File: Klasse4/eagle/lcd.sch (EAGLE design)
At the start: 3 parts

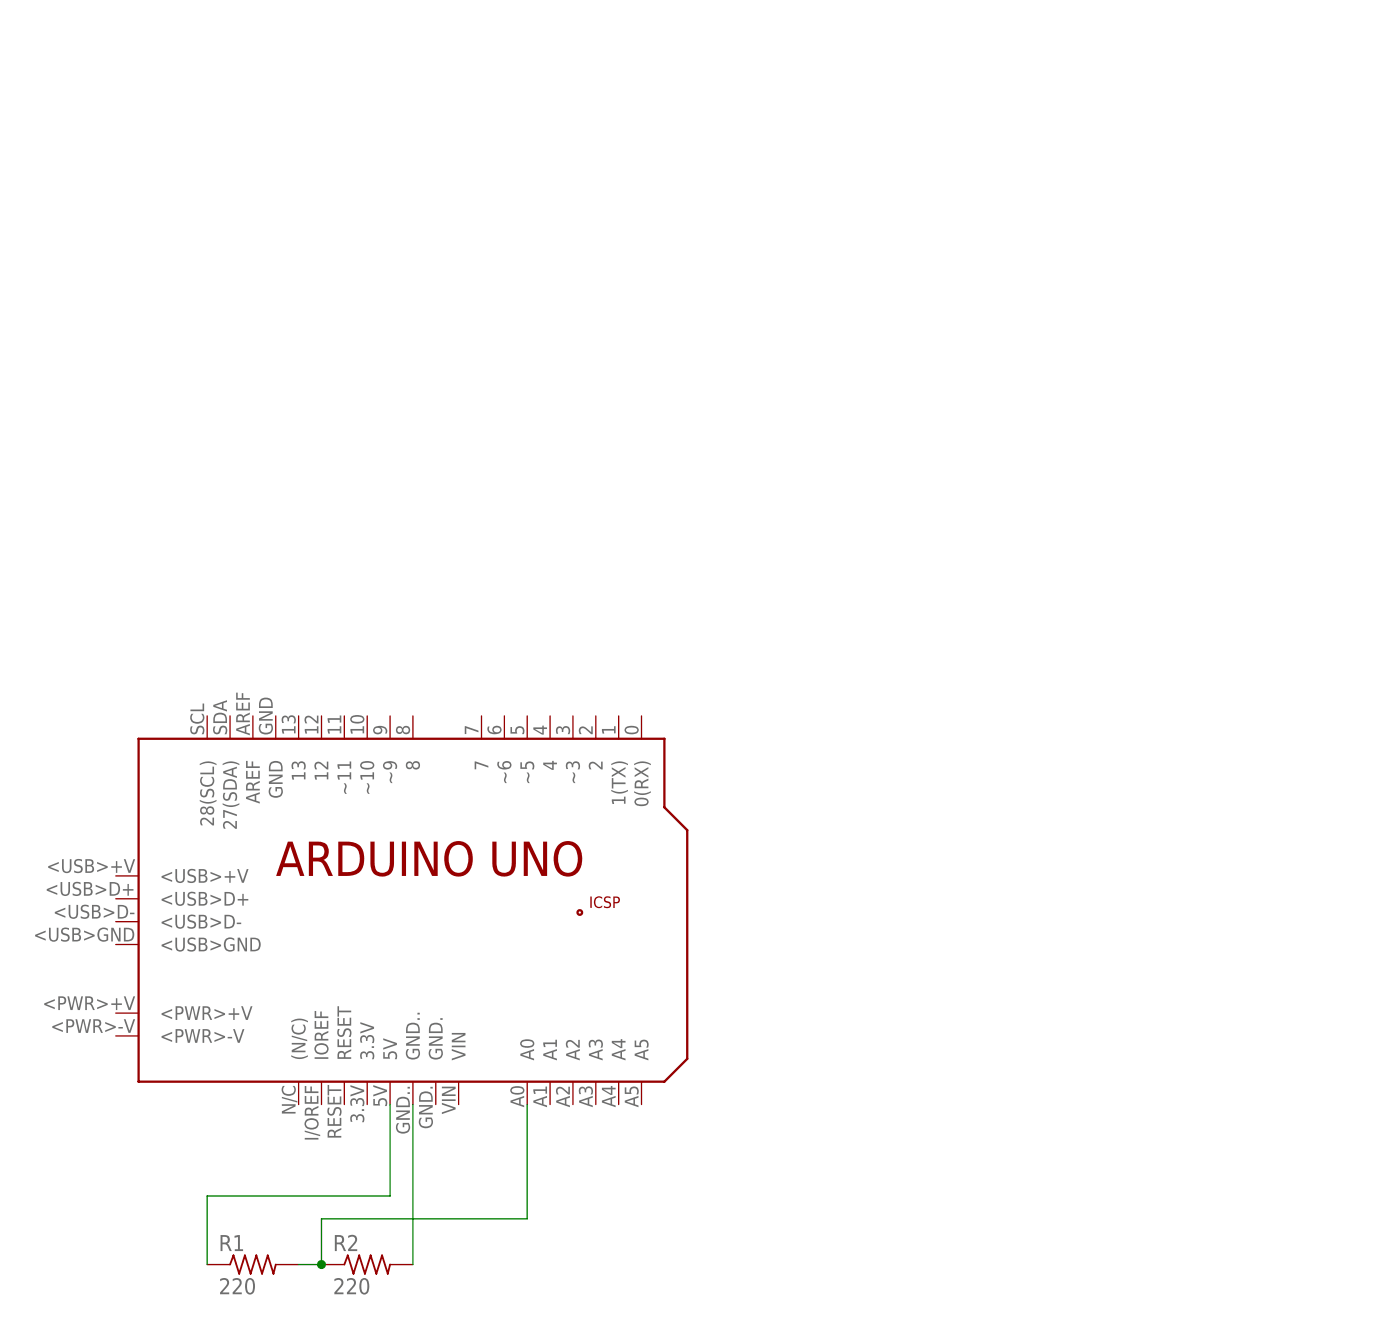
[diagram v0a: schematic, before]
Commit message: update
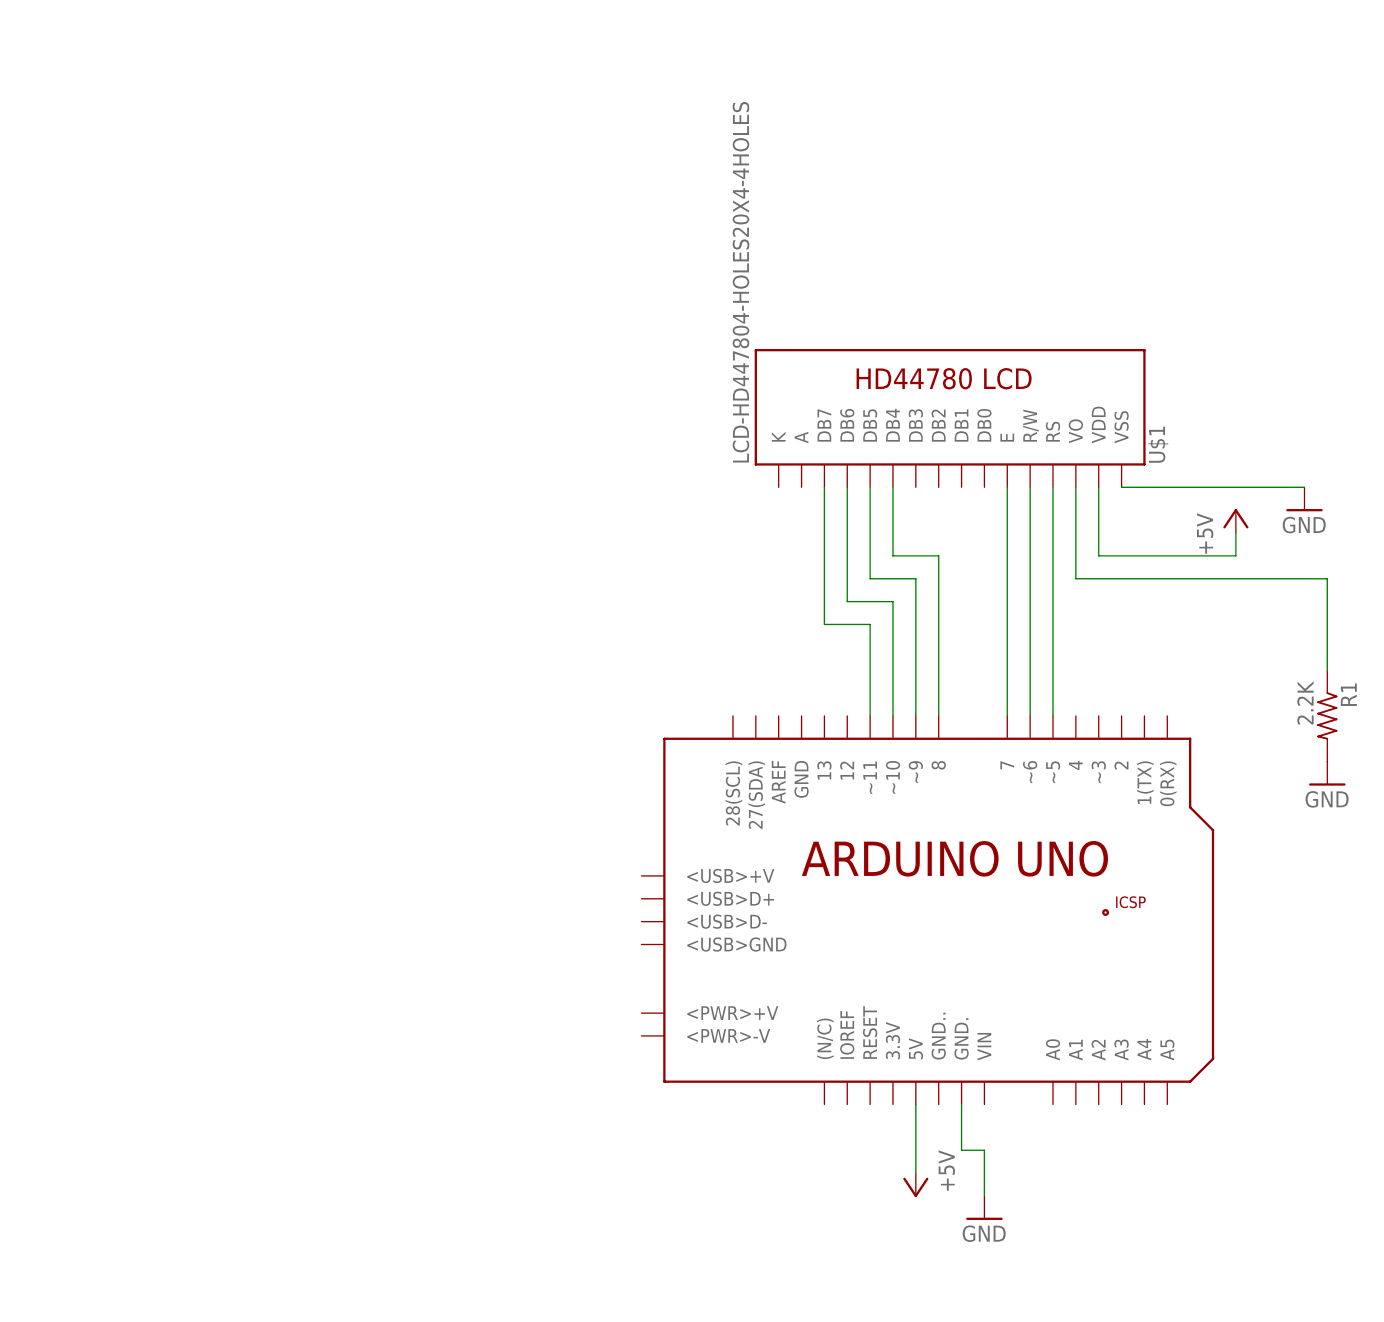
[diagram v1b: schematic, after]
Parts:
- removed R2: 220, resistor:R-US_0411/12
- added U$1: LCD-HD447804-HOLES20X4-4HOLES, HD44780LCD:LCD-HD447804-HOLES20X4-4HOLES
- PCB1: value ARDUINO_UNO -> ARDUINO_UNO_EXT; device E14_Arduino:ARDUINO_UNO -> E14_Arduino:ARDUINO_UNO_EXT
- R1: value 220 -> 2.2K; device resistor:R-US_0411/12 -> resistor:R-US_0204/5
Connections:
- new net +5V: PCB1.5V, U$1.VDD
- new net GND: PCB1.GND., R1.2
- new net N$4: R1.1, U$1.VO
- new net N$5: PCB1.~9, U$1.DB5
- new net N$6: PCB1.~10, U$1.DB6
- new net N$7: PCB1.~11, U$1.DB7
- new net N$9: PCB1.~5, U$1.RS
- net N$1: now also PCB1.8, U$1.DB4; no longer PCB1.A0, R1.2, R2.1
- net N$2: now also PCB1.~6, U$1.R/W; no longer R2.2
- net N$3: now also PCB1.7, U$1.E; no longer PCB1.5V, R1.1
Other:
- moved on the sheet: R1
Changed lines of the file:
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@@
 </classes>
 <parts>
-<part name="R1" library="resistor" deviceset="R-US_" device="0411/12" value="220"/>
-<part name="R2" library="resistor" deviceset="R-US_" device="0411/12" value="220"/>
-<part name="PCB1" library="E14_Arduino" deviceset="ARDUINO_UNO" device=""/>
+<part name="PCB1" library="E14_Arduino" deviceset="ARDUINO_UNO_EXT" device=""/>
+<part name="U$1" library="HD44780LCD" deviceset="LCD-HD44780" device="20X4-4HOLES" technology="4-HOLES"/>
+<part name="GND1" library="supply1" deviceset="GND" device=""/>
+<part name="P+1" library="supply1" deviceset="+5V" device=""/>
+<part name="GND2" library="supply1" deviceset="GND" device=""/>
+<part name="R1" library="resistor" deviceset="R-US_" device="0204/5" value="2.2K"/>
+<part name="P+2" library="supply1" deviceset="+5V" device=""/>
+<part name="GND3" library="supply1" deviceset="GND" device=""/>
 </parts>
 <sheets>
@@
 </plain>
 <instances>
-<instance part="R1" gate="G$1" x="-15.24" y="-10.16"/>
-<instance part="R2" gate="G$1" x="-2.54" y="-10.16"/>
-<instance part="PCB1" gate="G$1" x="2.54" y="30.48"/>
+<instance part="PCB1" gate="G$1" x="60.96" y="30.48"/>
+<instance part="U$1" gate="G$1" x="60.96" y="86.36" rot="MR90"/>
+<instance part="GND1" gate="1" x="101.6" y="73.66"/>
+<instance part="P+1" gate="1" x="93.98" y="73.66"/>
+<instance part="GND2" gate="1" x="104.14" y="43.18"/>
+<instance part="R1" gate="G$1" x="104.14" y="50.8" rot="R270"/>
+<instance part="P+2" gate="1" x="58.42" y="-2.54" rot="R180"/>
+<instance part="GND3" gate="1" x="66.04" y="-5.08"/>
 </instances>
 <busses>
 </busses>
 <nets>
-<net name="N$1" class="0">
+<net name="GND" class="0">
 <segment>
+<wire x1="81.28" y1="76.2" x2="101.6" y2="76.2" width="0.1524" layer="91"/>
+<pinref part="GND1" gate="1" pin="GND"/>
+</segment>
+<segment>
+<pinref part="GND2" gate="1" pin="GND"/>
 <pinref part="R1" gate="G$1" pin="2"/>
-<pinref part="R2" gate="G$1" pin="1"/>
-<wire x1="-7.62" y1="-10.16" x2="-10.16" y2="-10.16" width="0.1524" layer="91"/>
-<wire x1="-7.62" y1="-10.16" x2="-7.62" y2="-5.08" width="0.1524" layer="91"/>
-<junction x="-7.62" y="-10.16"/>
-<wire x1="-7.62" y1="-5.08" x2="15.24" y2="-5.08" width="0.1524" layer="91"/>
-<pinref part="PCB1" gate="G$1" pin="A0"/>
-<wire x1="15.24" y1="-5.08" x2="15.24" y2="7.62" width="0.1524" layer="91"/>
+</segment>
+<segment>
+<pinref part="PCB1" gate="G$1" pin="GND."/>
+<wire x1="63.5" y1="7.62" x2="63.5" y2="2.54" width="0.1524" layer="91"/>
+<wire x1="63.5" y1="2.54" x2="66.04" y2="2.54" width="0.1524" layer="91"/>
+<wire x1="66.04" y1="2.54" x2="66.04" y2="-2.54" width="0.1524" layer="91"/>
+<pinref part="GND3" gate="1" pin="GND"/>
+</segment>
+</net>
+<net name="N$9" class="0">
+<segment>
+<pinref part="PCB1" gate="G$1" pin="~5"/>
+<pinref part="U$1" gate="G$1" pin="RS"/>
+<wire x1="73.66" y1="76.2" x2="73.66" y2="50.8" width="0.1524" layer="91"/>
+</segment>
+</net>
+<net name="+5V" class="0">
+<segment>
+<pinref part="U$1" gate="G$1" pin="VDD"/>
+<wire x1="78.74" y1="76.2" x2="78.74" y2="68.58" width="0.1524" layer="91"/>
+<wire x1="78.74" y1="68.58" x2="93.98" y2="68.58" width="0.1524" layer="91"/>
+<pinref part="P+1" gate="1" pin="+5V"/>
+<wire x1="93.98" y1="68.58" x2="93.98" y2="71.12" width="0.1524" layer="91"/>
+</segment>
+<segment>
+<pinref part="PCB1" gate="G$1" pin="5V"/>
+<pinref part="P+2" gate="1" pin="+5V"/>
+<wire x1="58.42" y1="7.62" x2="58.42" y2="0" width="0.1524" layer="91"/>
+</segment>
+</net>
+<net name="N$4" class="0">
+<segment>
+<pinref part="U$1" gate="G$1" pin="VO"/>
+<wire x1="76.2" y1="76.2" x2="76.2" y2="66.04" width="0.1524" layer="91"/>
+<wire x1="76.2" y1="66.04" x2="104.14" y2="66.04" width="0.1524" layer="91"/>
+<wire x1="104.14" y1="55.88" x2="104.14" y2="66.04" width="0.1524" layer="91"/>
+<pinref part="R1" gate="G$1" pin="1"/>
 </segment>
 </net>
 <net name="N$2" class="0">
 <segment>
-<pinref part="R2" gate="G$1" pin="2"/>
-<wire x1="2.54" y1="-10.16" x2="2.54" y2="7.62" width="0.1524" layer="91"/>
+<pinref part="U$1" gate="G$1" pin="R/W"/>
+<pinref part="PCB1" gate="G$1" pin="~6"/>
+<wire x1="71.12" y1="76.2" x2="71.12" y2="50.8" width="0.1524" layer="91"/>
 </segment>
 </net>
 <net name="N$3" class="0">
 <segment>
-<pinref part="PCB1" gate="G$1" pin="5V"/>
-<wire x1="0" y1="7.62" x2="0" y2="-2.54" width="0.1524" layer="91"/>
-<wire x1="0" y1="-2.54" x2="-20.32" y2="-2.54" width="0.1524" layer="91"/>
-<pinref part="R1" gate="G$1" pin="1"/>
-<wire x1="-20.32" y1="-2.54" x2="-20.32" y2="-10.16" width="0.1524" layer="91"/>
+<pinref part="U$1" gate="G$1" pin="E"/>
+<pinref part="PCB1" gate="G$1" pin="7"/>
+<wire x1="68.58" y1="76.2" x2="68.58" y2="50.8" width="0.1524" layer="91"/>
 </segment>
 </net>
+<net name="N$1" class="0">
+<segment>
+<pinref part="U$1" gate="G$1" pin="DB4"/>
+<wire x1="55.88" y1="76.2" x2="55.88" y2="68.58" width="0.1524" layer="91"/>
+<pinref part="PCB1" gate="G$1" pin="8"/>
+<wire x1="55.88" y1="68.58" x2="60.96" y2="68.58" width="0.1524" layer="91"/>
+<wire x1="60.96" y1="68.58" x2="60.96" y2="50.8" width="0.1524" layer="91"/>
+</segment>
+</net>
+<net name="N$5" class="0">
+<segment>
+<pinref part="PCB1" gate="G$1" pin="~9"/>
+<wire x1="58.42" y1="50.8" x2="58.42" y2="66.04" width="0.1524" layer="91"/>
+<wire x1="58.42" y1="66.04" x2="53.34" y2="66.04" width="0.1524" layer="91"/>
+<pinref part="U$1" gate="G$1" pin="DB5"/>
+<wire x1="53.34" y1="66.04" x2="53.34" y2="76.2" width="0.1524" layer="91"/>
+</segment>
+</net>
+<net name="N$6" class="0">
+<segment>
+<pinref part="U$1" gate="G$1" pin="DB6"/>
+<wire x1="50.8" y1="76.2" x2="50.8" y2="63.5" width="0.1524" layer="91"/>
+<wire x1="50.8" y1="63.5" x2="55.88" y2="63.5" width="0.1524" layer="91"/>
+<pinref part="PCB1" gate="G$1" pin="~10"/>
+<wire x1="55.88" y1="63.5" x2="55.88" y2="50.8" width="0.1524" layer="91"/>
+</segment>
+</net>
+<net name="N$7" class="0">
+<segment>
+<pinref part="PCB1" gate="G$1" pin="~11"/>
+<wire x1="53.34" y1="50.8" x2="53.34" y2="60.96" width="0.1524" layer="91"/>
+<wire x1="53.34" y1="60.96" x2="48.26" y2="60.96" width="0.1524" layer="91"/>
+<pinref part="U$1" gate="G$1" pin="DB7"/>
+<wire x1="48.26" y1="60.96" x2="48.26" y2="76.2" width="0.1524" layer="91"/>
+</segment>
+</net>
